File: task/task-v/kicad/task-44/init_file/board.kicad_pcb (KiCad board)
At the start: 2 copper layers, 55 x 30 mm, 0 parts

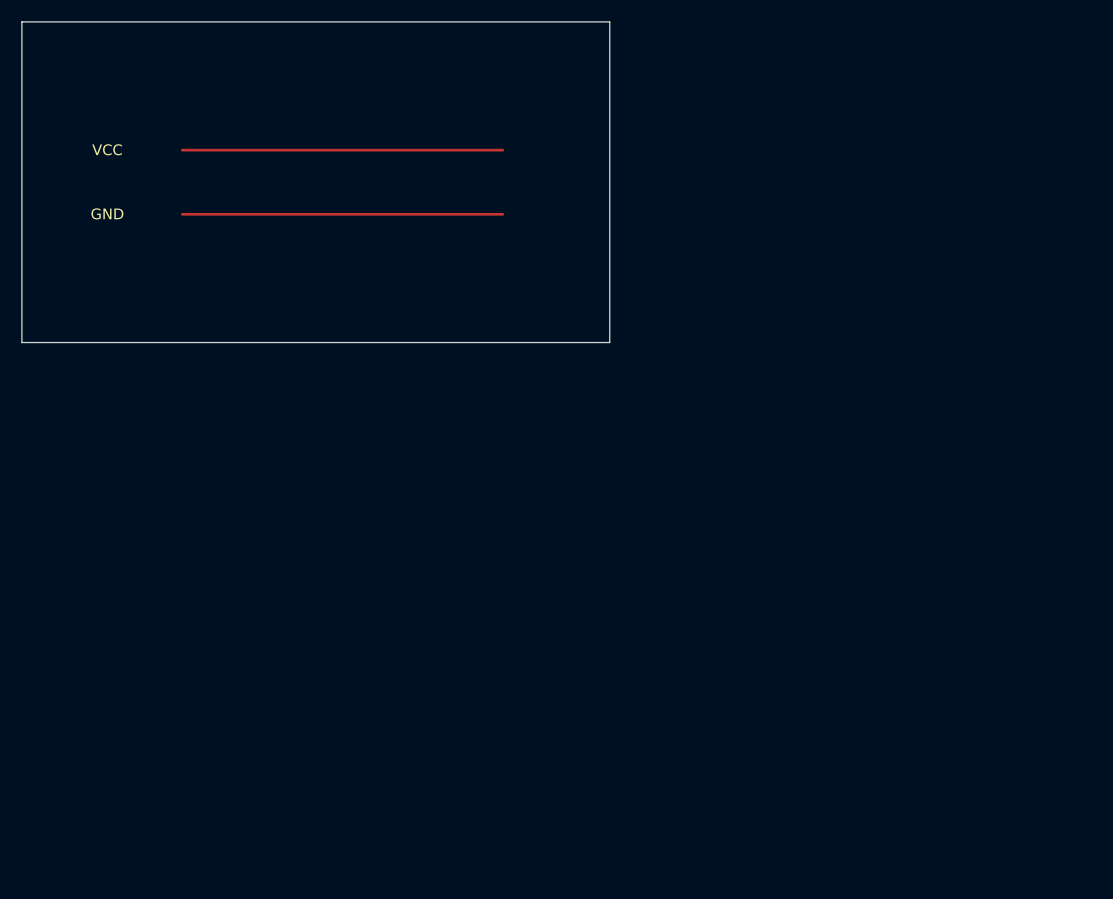
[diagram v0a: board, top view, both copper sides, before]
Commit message: Refine engineering task metadata and instructions
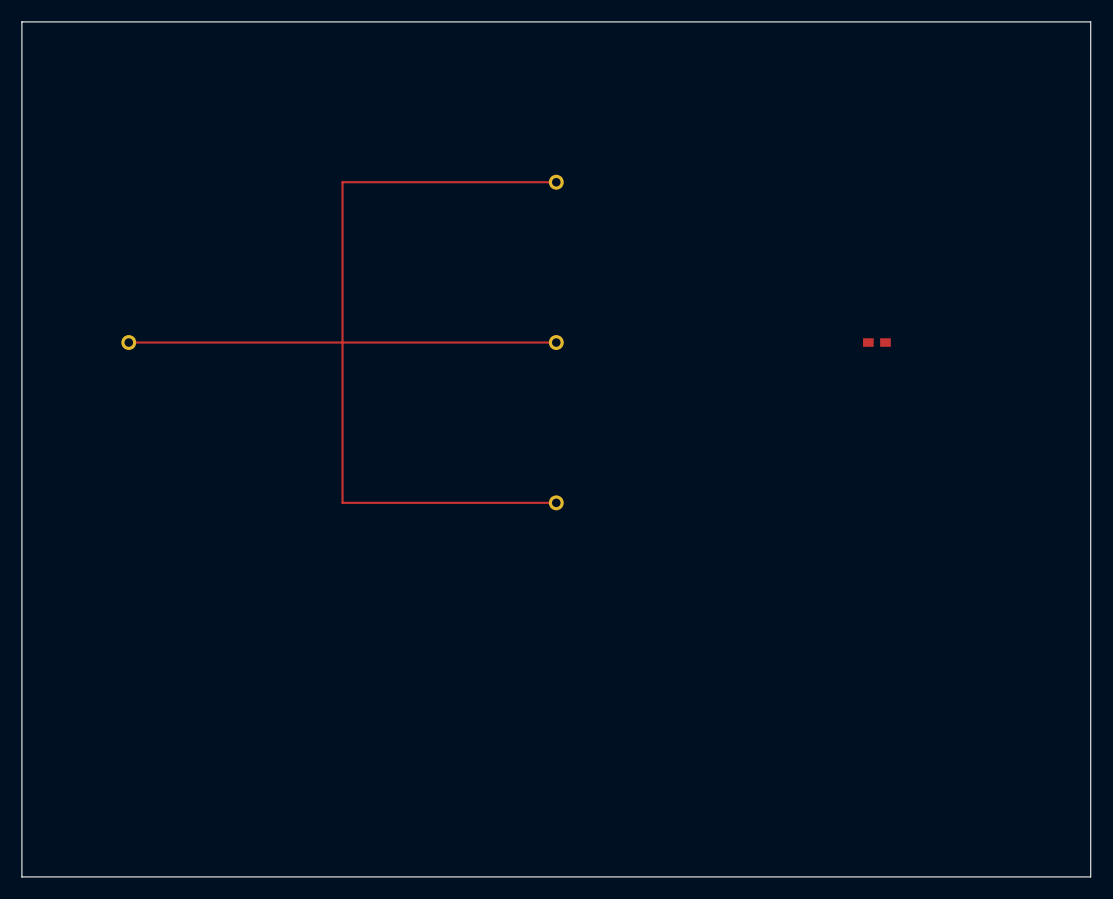
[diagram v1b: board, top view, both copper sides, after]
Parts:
- added ?: , Package_SO:SOIC-8_3.9x4.9mm_P1.27mm, F.Cu at (10.0, 30.0)
- added ?: , Package_SO:SOIC-8_3.9x4.9mm_P1.27mm, F.Cu at (50.0, 15.0)
- added ?: , Package_SO:SOIC-8_3.9x4.9mm_P1.27mm, F.Cu at (50.0, 30.0)
- added ?: , Package_SO:SOIC-8_3.9x4.9mm_P1.27mm, F.Cu at (50.0, 45.0)
- added ?: , Resistor_SMD:R_0603_1608Metric, F.Cu at (80.0, 30.0)
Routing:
- net CLK: track 0.00 -> 110.0 mm
- net VCC: track 30.0 -> 0.00 mm
- net GND: track 30.0 -> 0.00 mm
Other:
- board size 55 x 30 mm -> 100 x 80 mm
- rule pad_to_mask_clearance: 0.051 -> 0.1
- board text removed: "FAB NOTE"
- board text removed: "GND"
- board text removed: "VCC"
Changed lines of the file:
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@@
   (version 20240108)
   (generator "pcbnew")
-  (general (thickness 1.6) (legacy_teardrops no))
+  (generator_version "9.0")
+  (general
+    (thickness 1.6)
+    (legacy_teardrops no)
+  )
   (paper "A4")
   (layers
     (0 "F.Cu" signal)
     (31 "B.Cu" signal)
-    (37 "F.SilkS" user "F.Silkscreen")
     (44 "Edge.Cuts" user)
-    (47 "F.CrtYd" user "F.Courtyard")
-    (49 "F.Fab" user)
   )
-  (setup (pad_to_mask_clearance 0.051))
+  (setup
+    (pad_to_mask_clearance 0.1)
+    (allow_soldermask_bridges_in_footprints no)
+  )
   (net 0 "")
-  (net 1 "VCC")
+  (net 1 "CLK")
   (net 2 "GND")
-  (gr_text "VCC" (at 8 12 0) (layer "F.SilkS")
-    (effects (font (size 1 1) (thickness 0.15)))
+  (net 3 "VCC")
+  ; Source IC: U1 at (10, 30) — output pad drives CLK
+  (footprint "Package_SO:SOIC-8_3.9x4.9mm_P1.27mm" (layer "F.Cu") (at 10 30)
+    (reference "U1") (value "74HC04")
+    (pad "3" thru_hole circle (at 0 0) (size 1.4 1.4) (drill 0.8)
+      (layers "F.Cu" "B.Cu" "F.Mask" "B.Mask") (net 1 "CLK"))
   )
-  (gr_text "GND" (at 8 18 0) (layer "F.SilkS")
-    (effects (font (size 1 1) (thickness 0.15)))
+  ; Load 1: U2 at (50, 15)
+  (footprint "Package_SO:SOIC-8_3.9x4.9mm_P1.27mm" (layer "F.Cu") (at 50 15)
+    (reference "U2") (value "74HCT74")
+    (pad "1" thru_hole circle (at 0 0) (size 1.4 1.4) (drill 0.8)
+      (layers "F.Cu" "B.Cu" "F.Mask" "B.Mask") (net 1 "CLK"))
   )
-  (gr_text "FAB NOTE" (at 26 6 0) (layer "F.Fab")
-    (effects (font (size 1 1) (thickness 0.15)))
+  ; Load 2: U3 at (50, 30)
+  (footprint "Package_SO:SOIC-8_3.9x4.9mm_P1.27mm" (layer "F.Cu") (at 50 30)
+    (reference "U3") (value "74HCT74")
+    (pad "1" thru_hole circle (at 0 0) (size 1.4 1.4) (drill 0.8)
+      (layers "F.Cu" "B.Cu" "F.Mask" "B.Mask") (net 1 "CLK"))
   )
-  (gr_rect (start 12 8) (end 48 22) (layer "F.CrtYd") (width 0.1))
-  (segment (start 15 12) (end 45 12) (width 0.25) (layer "F.Cu") (net 1))
-  (segment (start 15 18) (end 45 18) (width 0.25) (layer "F.Cu") (net 2))
-  (gr_rect (start 0 0) (end 55 30) (layer "Edge.Cuts") (width 0.05))
+  ; Load 3: U4 at (50, 45)
+  (footprint "Package_SO:SOIC-8_3.9x4.9mm_P1.27mm" (layer "F.Cu") (at 50 45)
+    (reference "U4") (value "74HCT74")
+    (pad "1" thru_hole circle (at 0 0) (size 1.4 1.4) (drill 0.8)
+      (layers "F.Cu" "B.Cu" "F.Mask" "B.Mask") (net 1 "CLK"))
+  )
+  ; Series termination resistor placeholder (scratch area, not connected)
+  (footprint "Resistor_SMD:R_0603_1608Metric" (layer "F.Cu") (at 80 30)
+    (reference "R_TERM") (value "22R")
+    (pad "1" smd rect (at -0.8 0) (size 1.0 0.8)
+      (layers "F.Cu" "F.Paste" "F.Mask") (net 0 ""))
+    (pad "2" smd rect (at 0.8 0) (size 1.0 0.8)
+      (layers "F.Cu" "F.Paste" "F.Mask") (net 0 ""))
+  )
+  ; Star topology tracks: source (10,30) -> hub (30,30)
+  (segment (start 10 30) (end 30 30) (width 0.2) (layer "F.Cu") (net 1))
+  ; Hub (30,30) -> U2 (50,15)
+  (segment (start 30 30) (end 30 15) (width 0.2) (layer "F.Cu") (net 1))
+  (segment (start 30 15) (end 50 15) (width 0.2) (layer "F.Cu") (net 1))
+  ; Hub (30,30) -> U3 (50,30)
+  (segment (start 30 30) (end 50 30) (width 0.2) (layer "F.Cu") (net 1))
+  ; Hub (30,30) -> U4 (50,45)
+  (segment (start 30 30) (end 30 45) (width 0.2) (layer "F.Cu") (net 1))
+  (segment (start 30 45) (end 50 45) (width 0.2) (layer "F.Cu") (net 1))
+  (gr_rect (start 0 0) (end 100 80) (layer "Edge.Cuts") (width 0.1))
 )
